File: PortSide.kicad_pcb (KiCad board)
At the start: 2 copper layers, 67.5 x 59.5 mm, 32 parts, among them J1 Conn_ARM_JTAG_SWD_10, J2 USB_C_Receptacle_USB2.0_14P, J3 Conn_01x14, J4 Conn_02x08_Top_Bottom, Q1 2N7002, Q2 MMDT3904, U1 TCAN3404, U2 ESP32-S3-WROOM-1, U3 AP2112K-3.3, U4 INA226, U5 LM5164DDA, U7 CP2102N-Axx-xQFN24

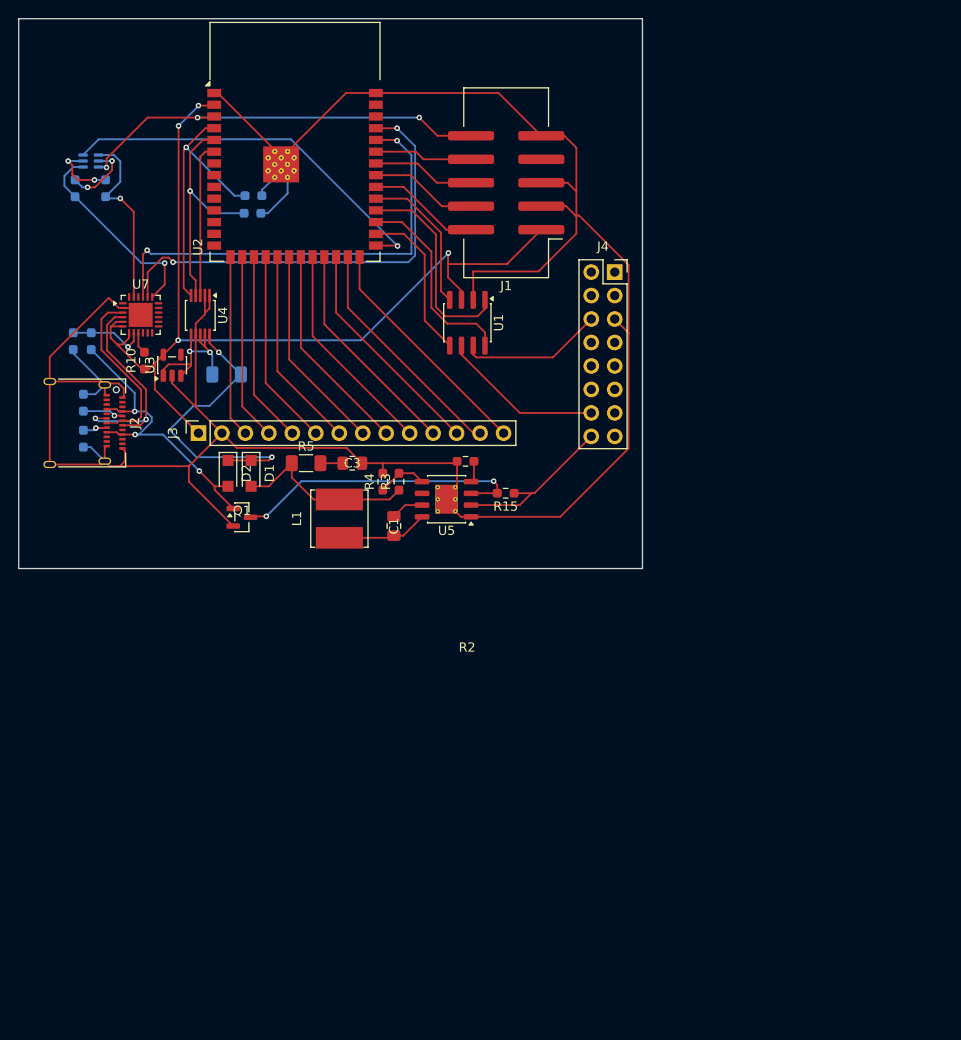
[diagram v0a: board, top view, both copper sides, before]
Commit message: Version 2, still not happy with that
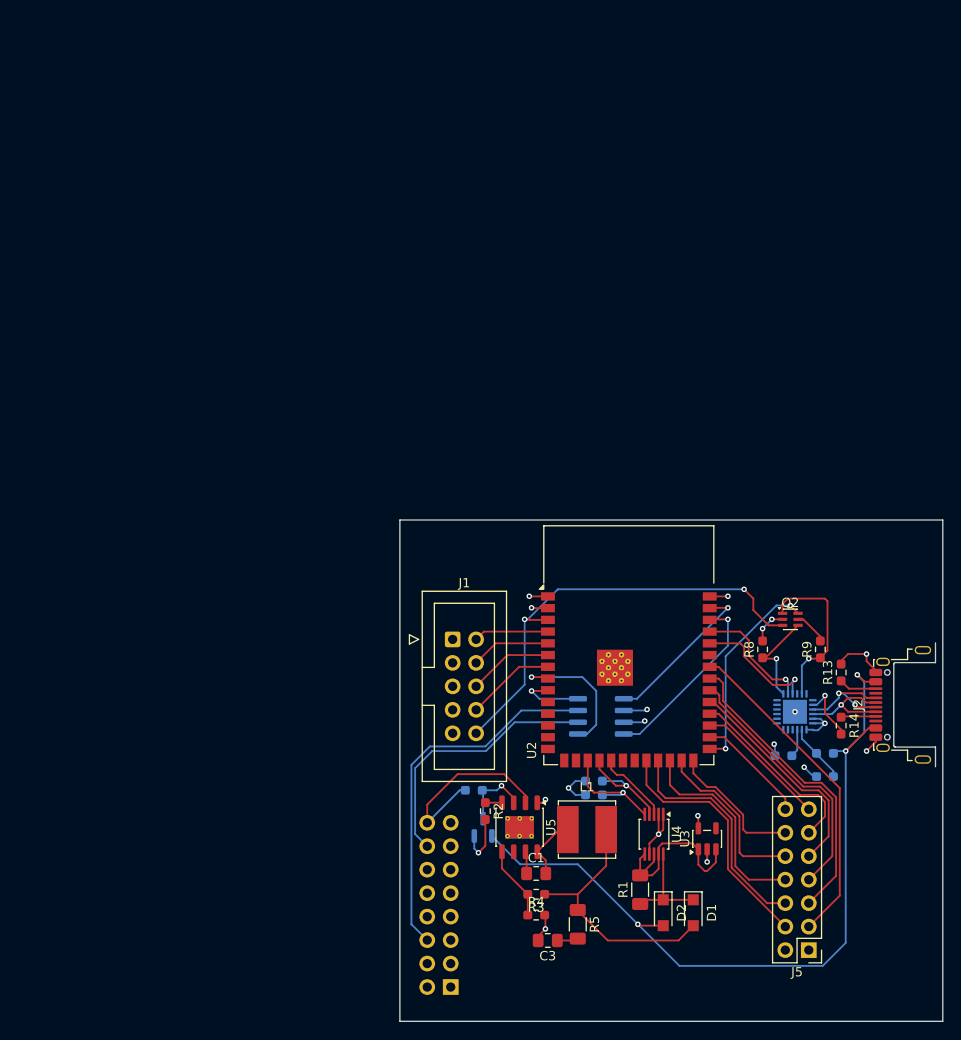
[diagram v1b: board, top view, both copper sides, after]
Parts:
- removed J3: Conn_01x14, Connector_PinSocket_2.54mm:PinSocket_1x14_P2.54mm_Vertical
- added J5: Conn_02x07_Counter_Clockwise, Connector_PinHeader_2.54mm:PinHeader_2x07_P2.54mm_Vertical, F.Cu at (155.5, 155.8)
- J1: footprint Connector_IDC:IDC-Header_2x05_P2.54mm_Vertical_SMD -> Connector_IDC:IDC-Header_2x05_P2.54mm_Vertical
- J2: footprint Connector_USB:USB_C_Receptacle_Amphenol_12401610E4-2A -> Connector_USB:USB_C_Receptacle_Amphenol_12401948E412A
- J4, Q1, R10, R15, U1, U7: moved to B.Cu
- Q2, R1, R13, R14, R8, R9: moved to F.Cu
- moved J2 96.6 mm to (167.8, 129.2), turned to 90 degrees
- moved R12 94.0 mm to (157.2, 137.0), turned to 180 degrees
- moved R9 92.0 mm to (156.8, 123.2)
- moved R11 91.1 mm to (157.2, 134.5), turned to 180 degrees
- moved Q2 90.5 mm to (153.5, 120.0), turned to 0 degrees
- moved R8 89.6 mm to (150.5, 123.2)
- moved R14 89.1 mm to (159.0, 131.5), turned to -90 degrees
- moved R13 85.8 mm to (159.0, 125.8), turned to 90 degrees
- moved U7 82.8 mm to (154.0, 130.0), turned to 180 degrees
- moved R10 81.3 mm to (152.8, 134.8), turned to 0 degrees
- moved J4 79.4 mm to (116.8, 159.8)
- moved U3 77.3 mm to (144.5, 143.8)
- moved U4 74.6 mm to (138.8, 143.2)
- moved R6 73.3 mm to (132.2, 137.5), turned to 180 degrees
- moved R7 73.0 mm to (132.2, 139.0), turned to 180 degrees
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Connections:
- R6 pad 1: /SCL -> /SDA
- R7 pad 1: /SDA -> /SCL
- U2 pad 15: /LCD_CS -> unconnected-(U2-IO3-Pad15)
- U2 pad 16: /LCD_RESET -> unconnected-(U2-IO46-Pad16)
- U2 pad 17: /LCD_DC -> /SCL
- U2 pad 18: /LCD_MOSI -> /SDA
- U2 pad 19: /LCD_SCK -> /INA226_ALERT
- U2 pad 20: /LCD_LED -> unconnected-(U2-IO12-Pad20)
- U2 pad 21: /LCD_MISO -> unconnected-(U2-IO13-Pad21)
- U2 pad 22: /LCD_T_CLK -> /LCD_RESET
- U2 pad 23: /LCD_T_CS -> /LCD_MOSI
- U2 pad 24: /LCD_T_DIN -> /LCD_LED
- U2 pad 25: /LCD_T_DO -> /LCD_T_CLK
- U2 pad 26: /LCD_T_IRQ -> /LCD_T_DIN
- U2 pad 28: /TCAN3404_SHDN -> /LCD_T_IRQ
- U2 pad 29: /TCAN3404_STB -> /LCD_T_DO
- U2 pad 30: /CAN_TXD -> /LCD_T_CS
- U2 pad 31: /CAN_RXD -> /LCD_MISO
- U2 pad 32: /MTMS -> /LCD_SCK
- U2 pad 33: /MTCK -> /LCD_DC
- U2 pad 34: /MTDO -> /LCD_CS
- U2 pad 35: /MTDI -> unconnected-(U2-IO42-Pad35)
- U2 pad 38: unconnected-(U2-IO2-Pad38) -> /CAN_RXD
- U2 pad 39: unconnected-(U2-IO1-Pad39) -> /CAN_TXD
- U2 pad 4: /SCL -> /MTMS
- U2 pad 5: /SDA -> /MTCK
- U2 pad 6: /INA226_ALERT -> /MTDO
- U2 pad 7: unconnected-(U2-IO7-Pad7) -> /MTDI
- U2 pad 8: unconnected-(U2-IO15-Pad8) -> /TCAN3404_SHDN
- U2 pad 9: unconnected-(U2-IO16-Pad9) -> /TCAN3404_STB
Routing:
- net GND: track 272.3 -> 45.7 mm, vias 0 -> 14
- net +3.3V: track 103.8 -> 12.0 mm, vias 4 -> 5
- net /USB_VBUS: track 35.5 -> 86.1 mm
- net /ESP_TX: track 49.7 -> 13.0 mm, vias 2 -> 1
- net /ESP_RX: track 49.2 -> 13.6 mm, vias 2 -> 1
- net /CANH: track 15.6 -> 40.1 mm
- net Net-(Q1-D): track 32.1 -> 7.79 mm, vias 2 -> 1
- net /5v_SOURCE: track 33.1 -> 10.9 mm, vias 2 -> 0
- net /ESP_IO0: track 41.9 -> 22.2 mm, vias 1 -> 2
- net /SCL: track 28.9 -> 12.6 mm
- net /LCD_CS: track 19.7 -> 35.9 mm
- net /TCAN3404_STB: track 21.7 -> 7.18 mm, vias 0 -> 1
- net /SDA: track 25.7 -> 11.6 mm
- net /LCD_T_IRQ: track 25.5 -> 12.1 mm
- net /LCD_DC: track 20.8 -> 32.8 mm
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- added copper zone on In2.Cu, net +3.3V
- added copper zone on In1.Cu, net GND
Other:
- board size 67.5 x 59.5 mm -> 58.8 x 54.2 mm
- copper layers 2 -> 4
